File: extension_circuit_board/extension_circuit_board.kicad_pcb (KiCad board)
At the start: 2 copper layers, 95 x 72 mm, 29 parts, among them J1 AE_MRUSB_DIP, J2 Jetson_Nano_GPIO, J3 PiOLED 2x3, J4 FeatherWing_DCmotor, J5 Jetson Nano Power, J6 Motor Power, SW1 SW_SPDT

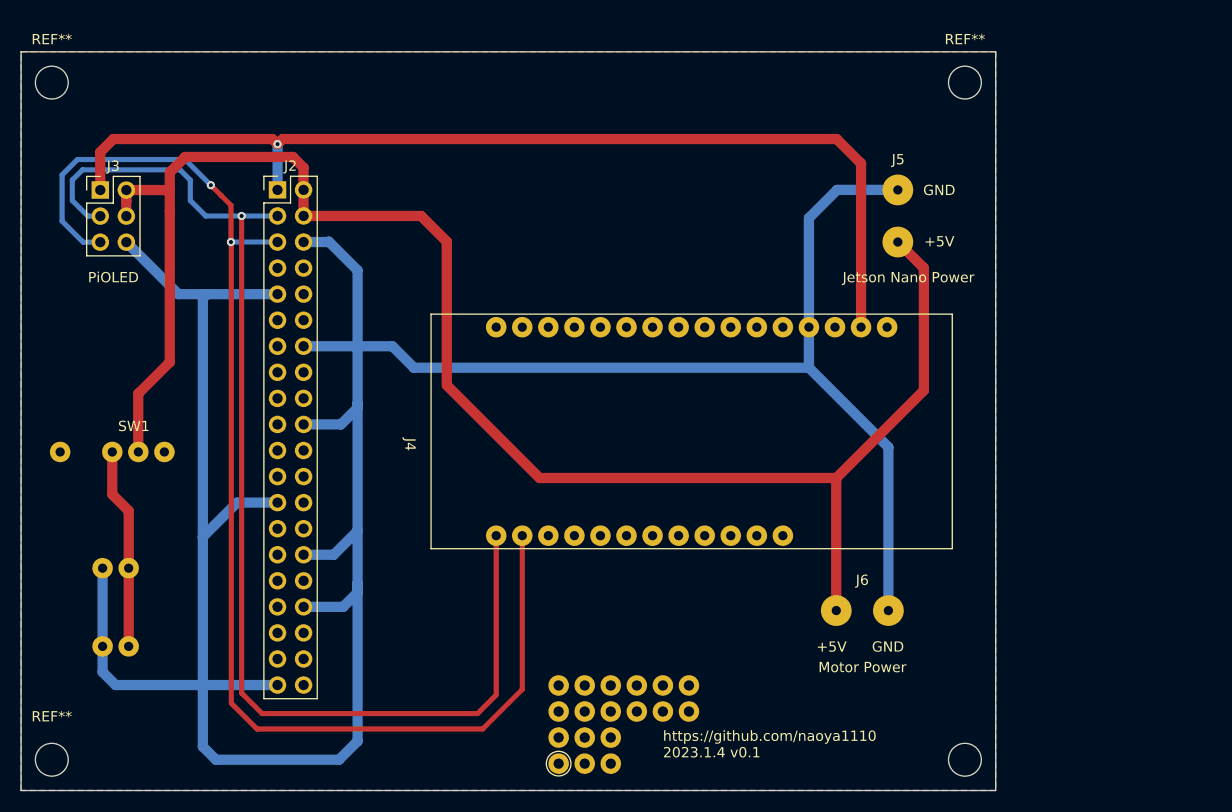
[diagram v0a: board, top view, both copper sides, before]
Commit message: updated
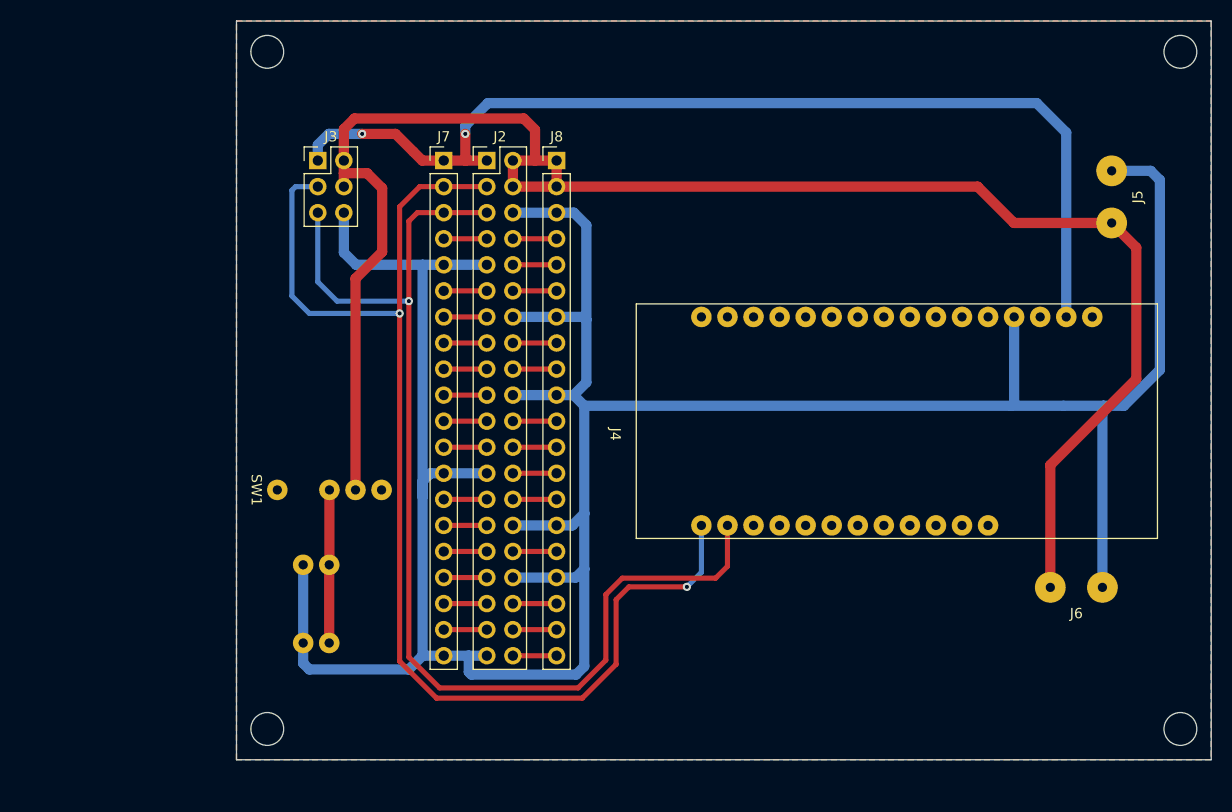
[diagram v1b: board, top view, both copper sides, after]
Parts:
- removed ? (x17): , 
- removed the REF** at (192.0, 119.0)
- removed the REF** at (103.0, 119.0)
- removed the REF** at (103.0, 53.0)
- removed the REF** at (152.4, 119.4)
- removed the REF** at (192.0, 53.0)
- added J7: GPIO_odd, Connector_PinHeader_2.54mm:PinHeader_1x20_P2.54mm_Vertical, F.Cu at (141.2, 60.6)
- added J8: GPIO_even, Connector_PinHeader_2.54mm:PinHeader_1x20_P2.54mm_Vertical, F.Cu at (152.2, 60.6)
- added REF**: MountingHole_3.2mm_M3, MountingHole:MountingHole_3.2mm_M3, F.Cu at (213.0, 50.0)
- added REF**: MountingHole_3.2mm_M3, MountingHole:MountingHole_3.2mm_M3, F.Cu at (124.0, 50.0)
- added REF**: MountingHole_3.2mm_M3, MountingHole:MountingHole_3.2mm_M3, F.Cu at (124.0, 116.0)
- added REF**: MountingHole_3.2mm_M3, MountingHole:MountingHole_3.2mm_M3, F.Cu at (213.0, 116.0)
- moved SW1 21.5 mm to (122.4, 92.7)
- moved J3 21.4 mm to (128.9, 60.6)
- moved J6 21.0 mm to (202.9, 104.7)
- moved J5 20.9 mm to (208.8, 64.1)
- moved J2 20.6 mm to (145.4, 60.6)
- moved J4 20.0 mm to (157.4, 87.3)
- moved J1 19.6 mm to (133.8, 103.8)
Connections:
- J2 pad 10: unconnected-(J2-Pad10) -> Net-(J2-Pad10)
- J2 pad 11: unconnected-(J2-Pad11) -> Net-(J2-Pad11)
- J2 pad 12: unconnected-(J2-Pad12) -> Net-(J2-Pad12)
- J2 pad 13: unconnected-(J2-Pad13) -> Net-(J2-Pad13)
- J2 pad 15: unconnected-(J2-Pad15) -> Net-(J2-Pad15)
- J2 pad 16: unconnected-(J2-Pad16) -> Net-(J2-Pad16)
- J2 pad 17: unconnected-(J2-Pad17) -> Net-(J2-Pad17)
- J2 pad 18: unconnected-(J2-Pad18) -> Net-(J2-Pad18)
- J2 pad 19: unconnected-(J2-Pad19) -> Net-(J2-Pad19)
- J2 pad 21: unconnected-(J2-Pad21) -> Net-(J2-Pad21)
- J2 pad 22: unconnected-(J2-Pad22) -> Net-(J2-Pad22)
- J2 pad 23: unconnected-(J2-Pad23) -> Net-(J2-Pad23)
- J2 pad 24: unconnected-(J2-Pad24) -> Net-(J2-Pad24)
- J2 pad 26: unconnected-(J2-Pad26) -> Net-(J2-Pad26)
- J2 pad 27: unconnected-(J2-Pad27) -> Net-(J2-Pad27)
- J2 pad 28: unconnected-(J2-Pad28) -> Net-(J2-Pad28)
- J2 pad 29: unconnected-(J2-Pad29) -> Net-(J2-Pad29)
- J2 pad 31: unconnected-(J2-Pad31) -> Net-(J2-Pad31)
- J2 pad 32: unconnected-(J2-Pad32) -> Net-(J2-Pad32)
- J2 pad 33: unconnected-(J2-Pad33) -> Net-(J2-Pad33)
- J2 pad 35: unconnected-(J2-Pad35) -> Net-(J2-Pad35)
- J2 pad 36: unconnected-(J2-Pad36) -> Net-(J2-Pad36)
- J2 pad 37: unconnected-(J2-Pad37) -> Net-(J2-Pad37)
- J2 pad 38: unconnected-(J2-Pad38) -> Net-(J2-Pad38)
- J2 pad 40: unconnected-(J2-Pad40) -> Net-(J2-Pad40)
- J2 pad 7: unconnected-(J2-Pad7) -> Net-(J2-Pad7)
- J2 pad 8: unconnected-(J2-Pad8) -> Net-(J2-Pad8)
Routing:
- net I2C_2_SCL: track 127.1 -> 111.8 mm, vias 2 -> 1
- net +5V: track 165.4 -> 172.1 mm
- net GND: track 286.8 -> 293.3 mm
- net I2C_2_SDA: track 117.2 -> 122.0 mm, vias 1 -> 2
- net Net-(J1-Pad3): track 19.6 -> 14.9 mm
- net Net-(J2-Pad8): track 0.00 -> 4.26 mm
- net Net-(J2-Pad40): track 0.00 -> 4.26 mm
- net Net-(J2-Pad38): track 0.00 -> 4.26 mm
- net Net-(J2-Pad36): track 0.00 -> 4.26 mm
- net Net-(J2-Pad32): track 0.00 -> 4.26 mm
- net Net-(J2-Pad28): track 0.00 -> 4.26 mm
- net Net-(J2-Pad26): track 0.00 -> 4.26 mm
- net Net-(J2-Pad24): track 0.00 -> 4.26 mm
- net Net-(J2-Pad22): track 0.00 -> 4.26 mm
- net Net-(J2-Pad18): track 0.00 -> 4.26 mm
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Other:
- board text removed: "+5V"
- board text removed: "GND"
- board text removed: "Jetson Nano Power"
- board text removed: "Motor Power"
- board text removed: "PiOLED"
- board text removed: "https://github.com/naoya1110 2023.1.4 v0.1"
